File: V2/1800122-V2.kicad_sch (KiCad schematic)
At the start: 34 parts, among them J1 USB_C_Receptacle_USB2.0_16P, J2 Conn_01x03, SW1 BOOTSEL, SW2 RESET, U1 W25Q128JVS, U2 NCP1117-3.3_SOT223, U3 RP2040, Y1 ABM8-272-T3

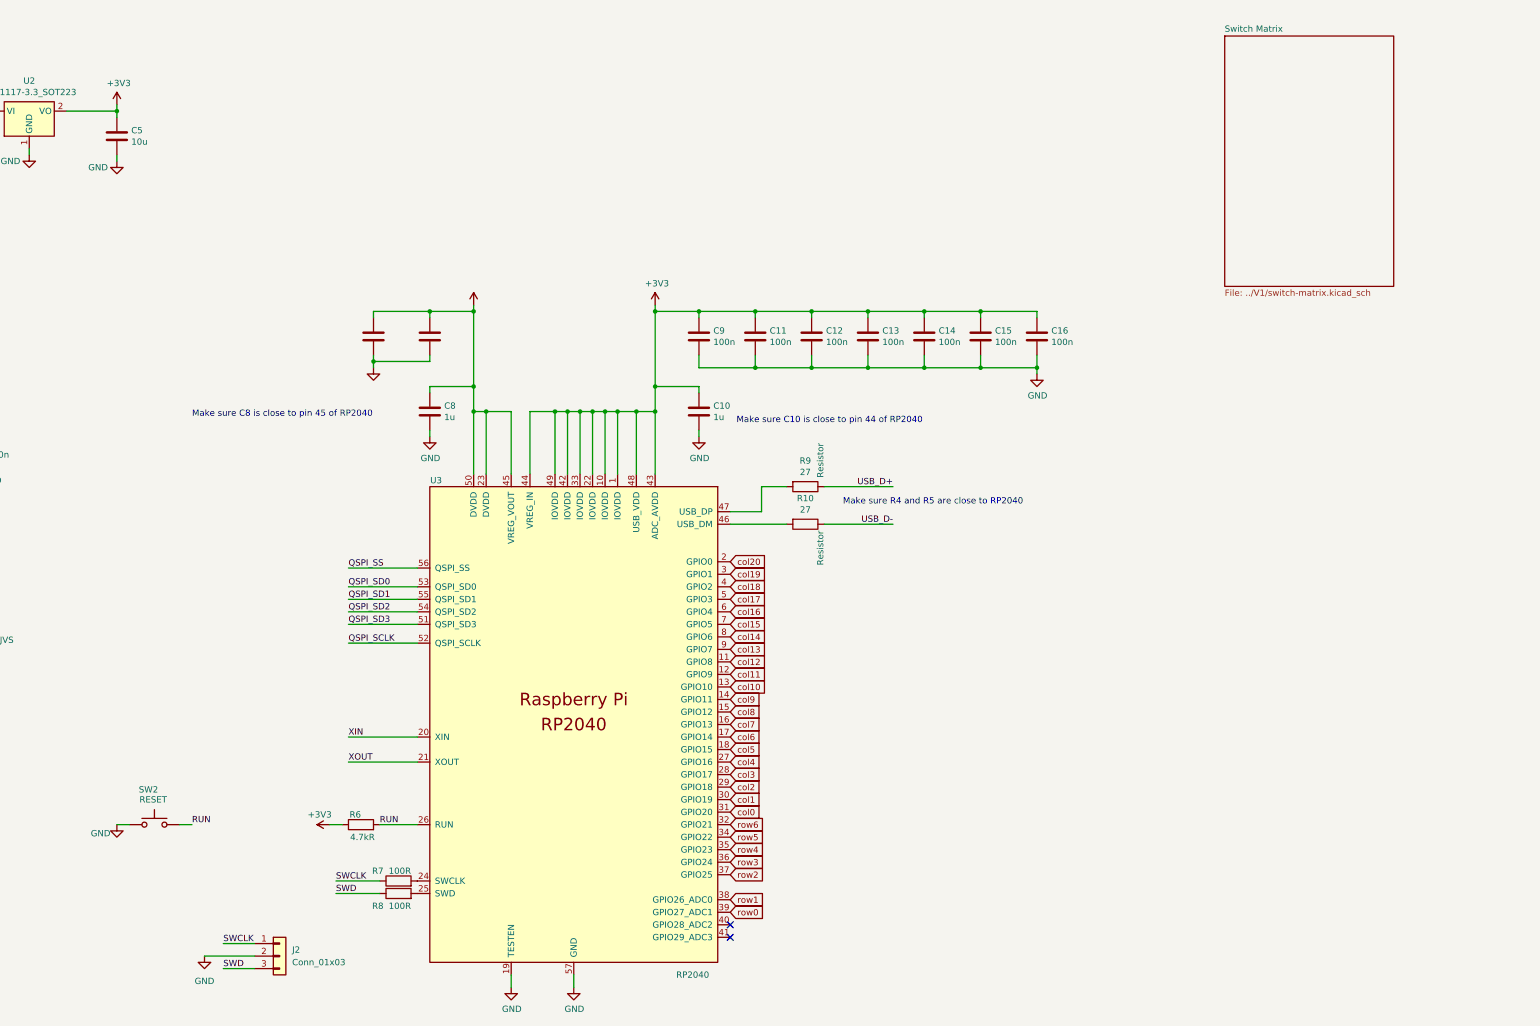
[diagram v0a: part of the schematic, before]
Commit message: Added updated KiCAD files with local repos
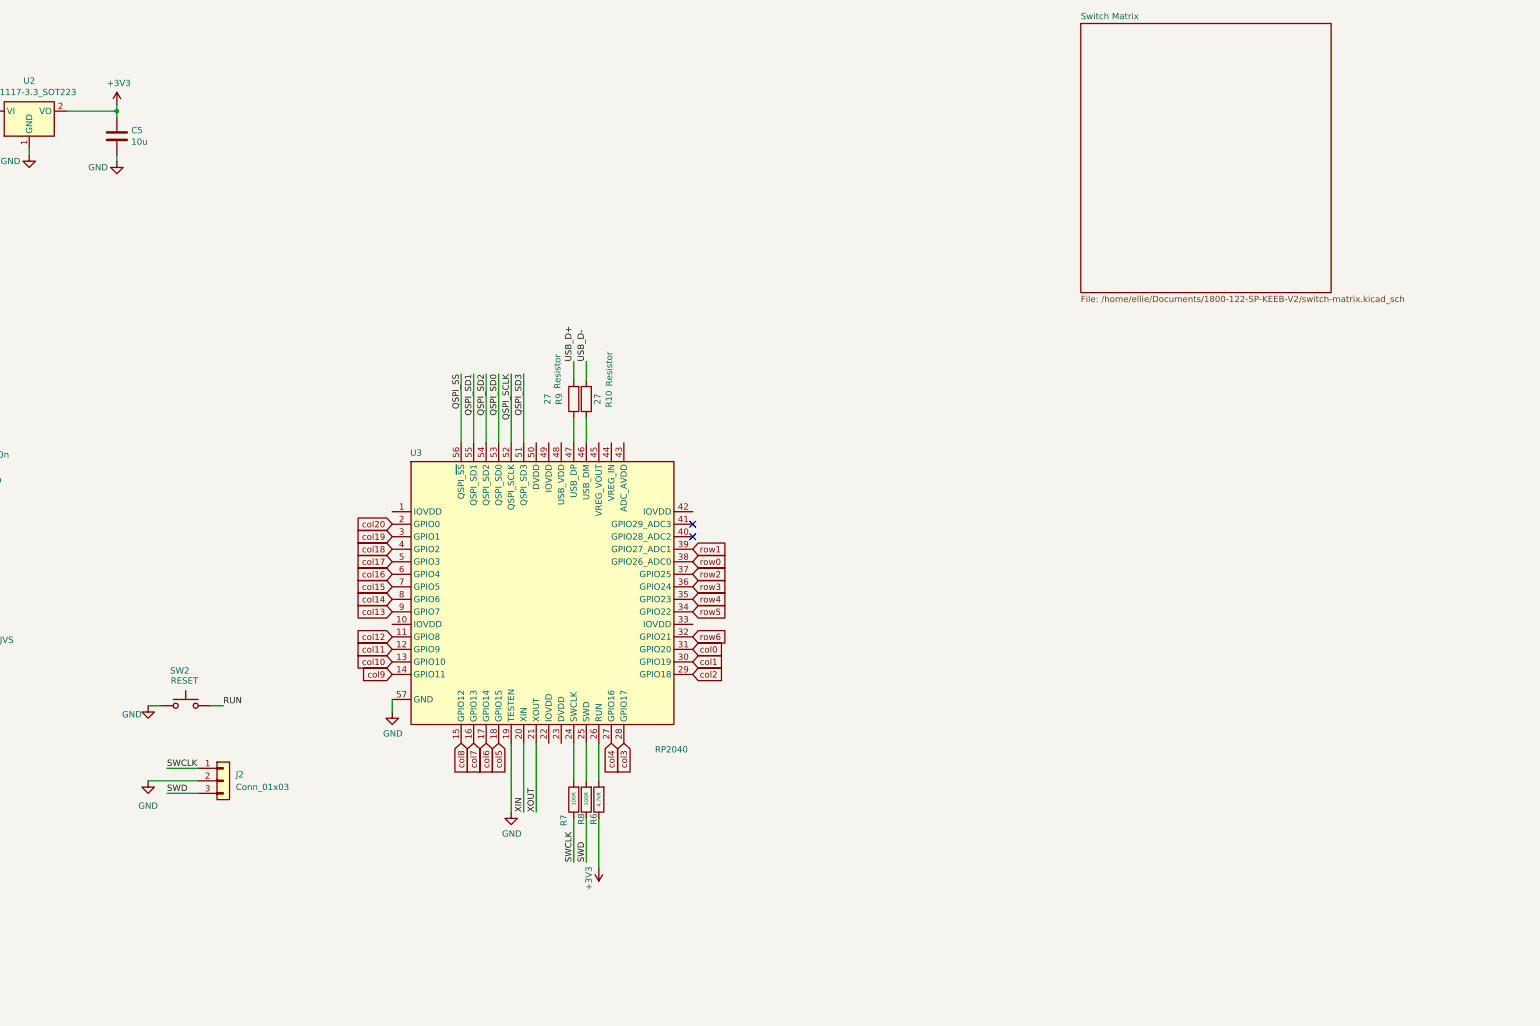
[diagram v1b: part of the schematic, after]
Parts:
- removed C10, C8: 1u, Capacitor_SMD:C_0402_1005Metric_Pad0.74x0.62mm_HandSolder, symbol Device:C
- removed C11, C12, C13, C14, C15, C16, C6, C7, C9: 100n, Capacitor_SMD:C_0402_1005Metric_Pad0.74x0.62mm_HandSolder, symbol Device:C
- removed U3: RP2040, RP2040:RP2040-QFN-56, symbol MCU_RaspberryPi_RP2040:RP2040
- added U3: RP2040, 122-LIB:RP2040, symbol 122-LIB:RP2040
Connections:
- net GND: now also U3.19 (TESTEN), U3.57 (GND)
- net QSPI_SCLK: now also U3.52 (QSPI_SCLK)
- net QSPI_SD0: now also U3.53 (QSPI_SD0)
- net QSPI_SD1: now also U3.55 (QSPI_SD1)
- net QSPI_SD2: now also U3.54 (QSPI_SD2)
- net QSPI_SD3: now also U3.51 (QSPI_SD3)
- net QSPI_SS: now also U3.56 (QSPI_~{SS})
- net RUN: no longer R6.2
- net USB_D+: now also R9.2; no longer R9.1
- net USB_D-: now also R10.2; no longer R10.1
- net XIN: now also U3.20 (XIN)
- net XOUT: now also U3.21 (XOUT)
- net col0: now also U3.31 (GPIO20)
- net col1: now also U3.30 (GPIO19)
- net col10: now also U3.13 (GPIO10)
- net col11: now also U3.12 (GPIO9)
- net col12: now also U3.11 (GPIO8)
- net col13: now also U3.9 (GPIO7)
- net col14: now also U3.8 (GPIO6)
- net col15: now also U3.7 (GPIO5)
- net col16: now also U3.6 (GPIO4)
- net col17: now also U3.5 (GPIO3)
- net col18: now also U3.4 (GPIO2)
- net col19: now also U3.3 (GPIO1)
- net col2: now also U3.29 (GPIO18)
- net col20: now also U3.2 (GPIO0)
- net col3: now also U3.28 (GPIO17)
- net col4: now also U3.27 (GPIO16)
- net col5: now also U3.18 (GPIO15)
- net col6: now also U3.17 (GPIO14)
- net col7: now also U3.16 (GPIO13)
- net col8: now also U3.15 (GPIO12)
- net col9: now also U3.14 (GPIO11)
- net row0: now also U3.38 (GPIO26_ADC0)
- net row1: now also U3.39 (GPIO27_ADC1)
- net row2: now also U3.37 (GPIO25)
- net row3: now also U3.36 (GPIO24)
- net row4: now also U3.35 (GPIO23)
- net row5: now also U3.34 (GPIO22)
- net row6: now also U3.32 (GPIO21)
- net at R7.2: now also U3.24 (SWCLK)
- net at R8.2: now also U3.25 (SWD)
- new net: R9.1, U3.47 (USB_DP)
- new net: R10.1, U3.46 (USB_DM)
- new net: R6.2, U3.26 (RUN)
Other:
- sheet Switch Matrix: file ../V1/switch-matrix.kicad_sch -> /home/ellie/Documents/1800-122-SP-KEEB-V2/switch-matrix.kicad_sch
- note removed: "Make sure C10 is close to pin 44 of RP2040"
- note removed: "Make sure C8 is close to pin 45 of RP2040"
- note removed: "Make sure R4 and R5 are close to RP2040"
- moved on the sheet: J2, R10, R6, R7, R8, R9, SW2
